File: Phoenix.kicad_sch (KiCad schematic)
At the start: 2 parts

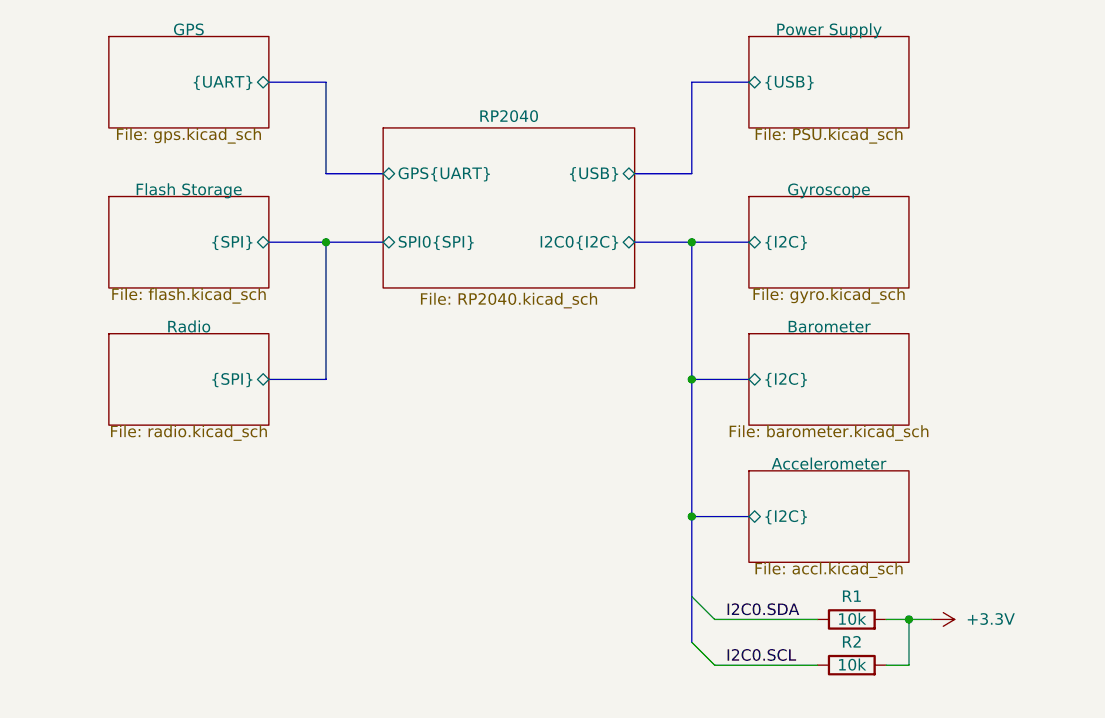
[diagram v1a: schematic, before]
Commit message: Various updates because I forgot to commit for a while
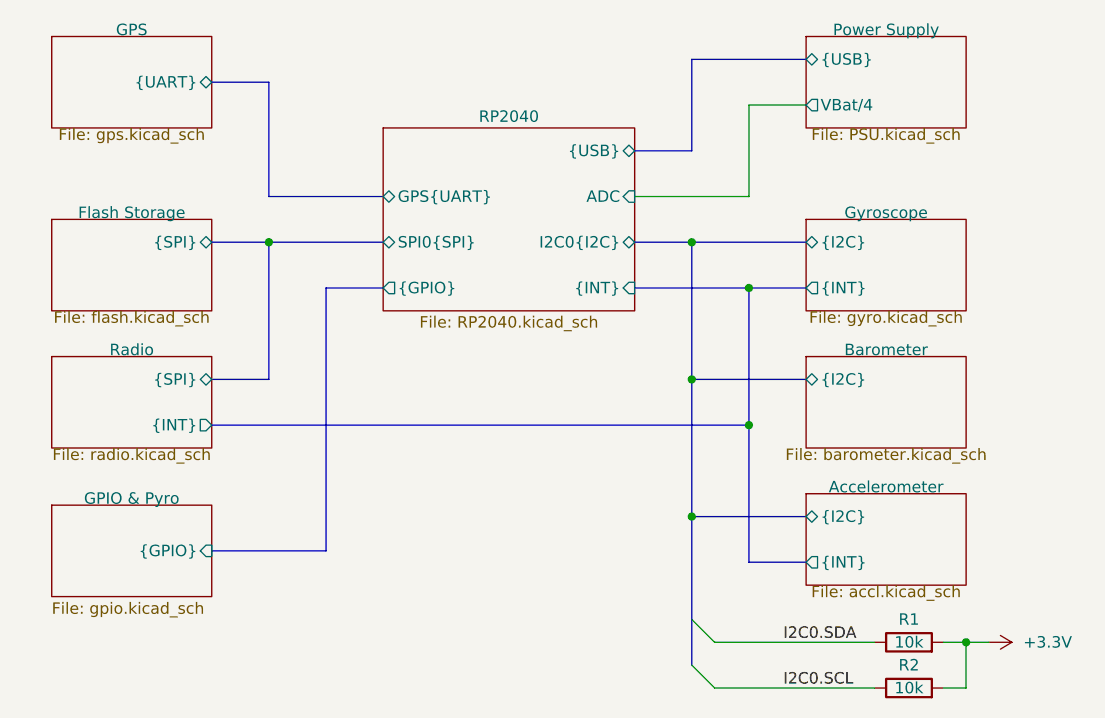
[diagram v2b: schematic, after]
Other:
- added sheet GPIO & Pyro (gpio.kicad_sch)
- sheet Accelerometer ports: added {INT}; removed none
- sheet Gyroscope ports: added {INT}; removed none
- sheet Power Supply ports: added VBat/4; removed none
- sheet RP2040 ports: added ADC, {GPIO}, {INT}; removed none
- sheet Radio ports: added {INT}; removed none
- moved on the sheet: R1, R2
